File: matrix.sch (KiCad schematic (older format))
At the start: 153 parts

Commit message: remap symbols.
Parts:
- D01, D02, D03, D04, D05, D06, D07, D08, D09, D10, D11, D12, D13, D14, D15, D16, D17, D18, D19, D21, D22, D23, D24, D26, D27, D28, D29, D30, D31, D32, D33, D34, D36, D37, D38, D39, D41, D42, D43, D44, D46, D47, D48, D49, D50, D51, D52, D53, D54, D55, D56, D57, D58, D59, D60, D61, D62, D63, D64, D65, D66, D67, D68, D69, D70: symbol DIODE -> device:DIODE
- DC1, DC2, DC3: symbol LED -> device:LED
- R4: symbol R -> device:R
- S01, S02, S03, S031, S04, S041, S05, S0512, S06, S07, S08, S09, S10, S101, S102, S11, S12, S13, S14, S15, S151, S16, S17, S18, S19, S21, S22, S23, S24, S26, S27, S28, S29, S30, S301, S302, S31, S32, S33, S34, S36, S37, S38, S39, S41, S42, S43, S44, S46, S47, S48, S49, S50, S51, S52, S53, S54, S55, S552, S56, S57, S58, S59, S60, S601, S602, S61, S62, S63, S64, S641, S65, S6512, S66, S661, S67, S68, S681, S682, S69, S691, S692, S70, S7012: symbol MX1A -> mx1a-simple:MX1A

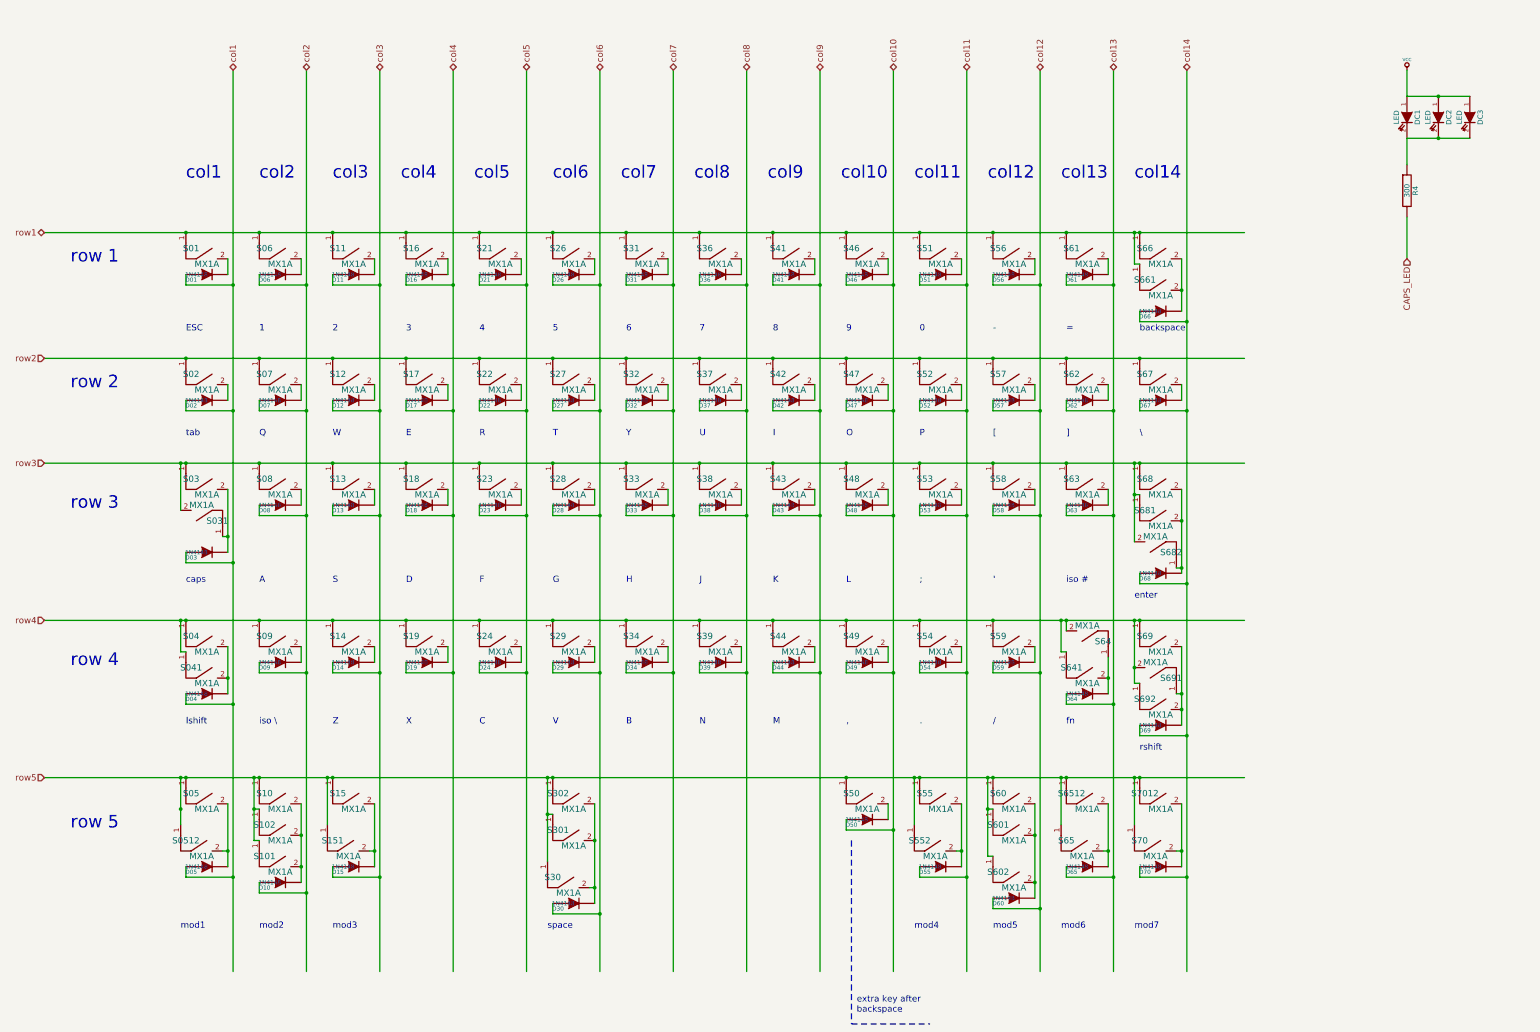
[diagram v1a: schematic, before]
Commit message: assign footprints.
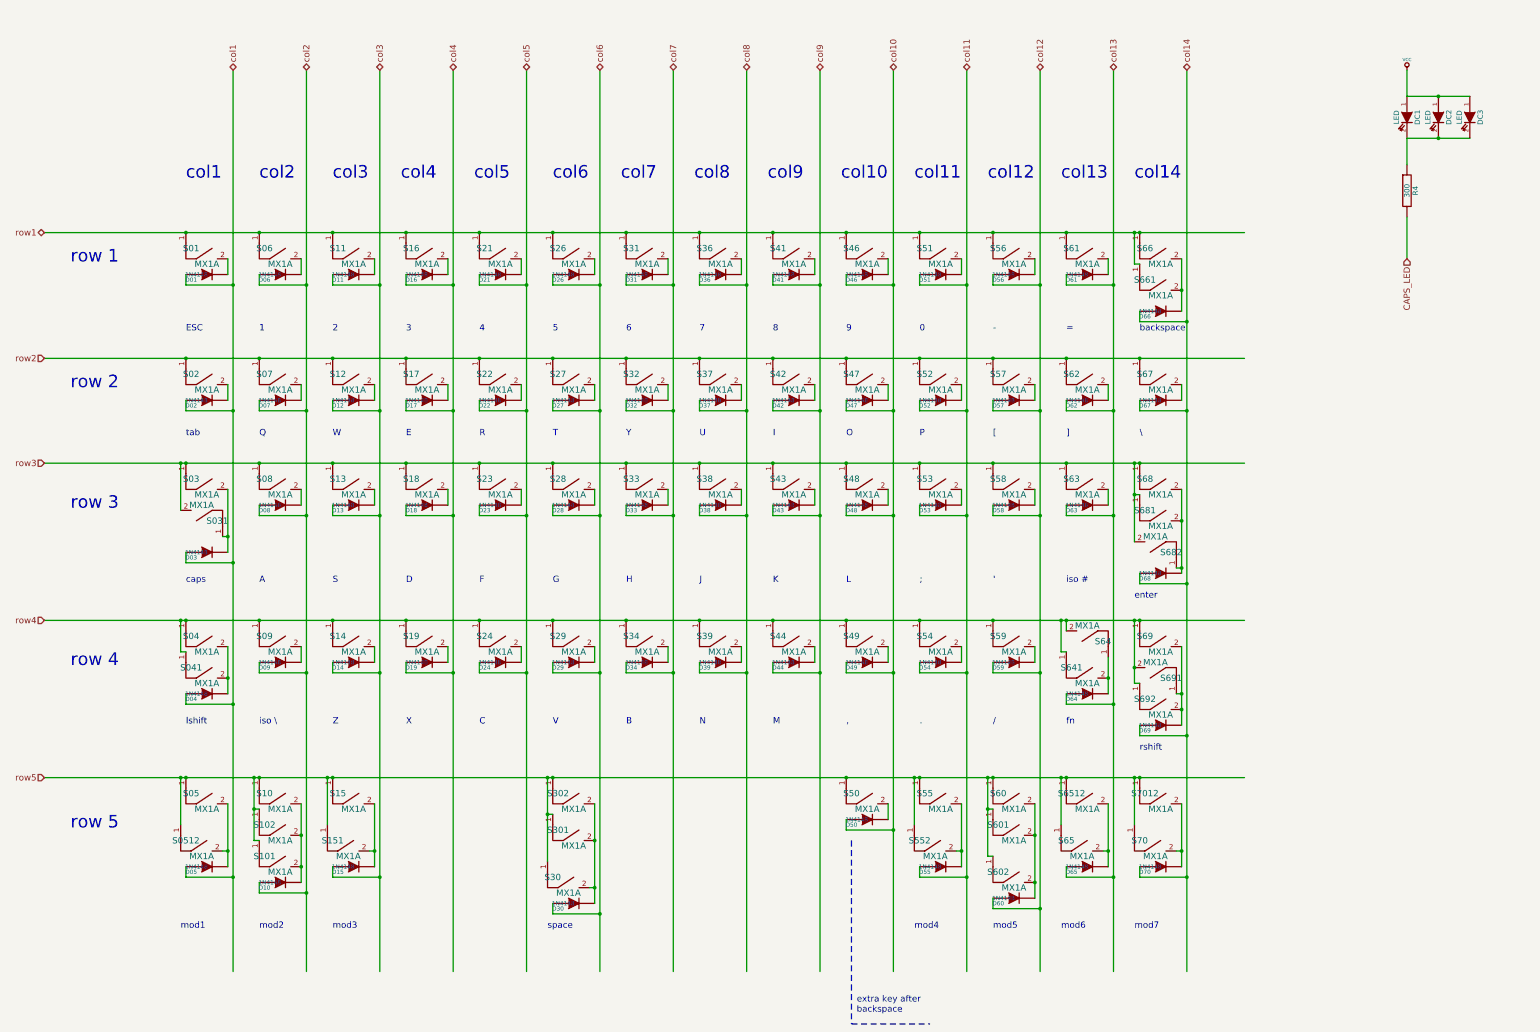
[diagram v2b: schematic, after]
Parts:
- DC3: footprint (none) -> mx1a:MX1A-led
- R4: footprint (none) -> res:resistor
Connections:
- wire segments 254 -> 423
